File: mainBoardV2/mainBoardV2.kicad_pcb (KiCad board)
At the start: 2 copper layers, 41.1 x 40.7 mm, 30 parts, among them J1 USB4125-GF-A_REVA2, U3 MCP73871-2AAI_ML, U4 MPU6050_Module, U5 TPS61023DRLT

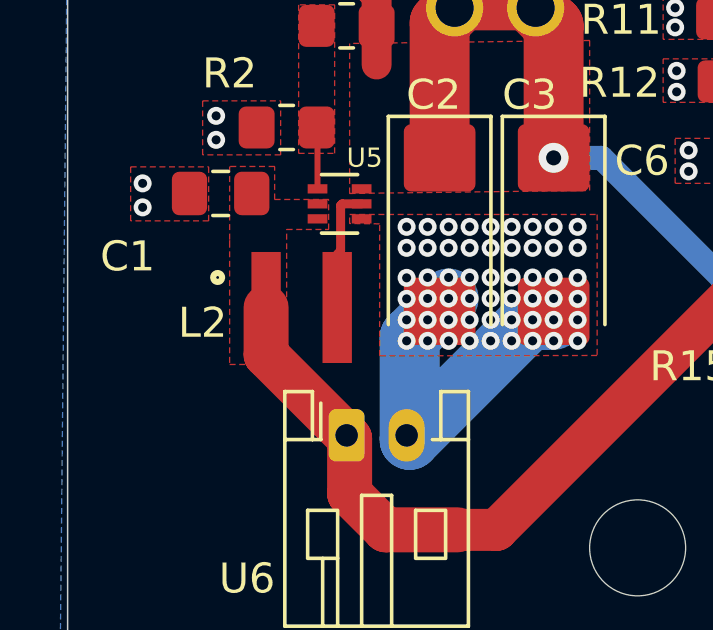
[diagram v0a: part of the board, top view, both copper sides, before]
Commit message: Revert "3.22.26.C1"
This reverts commit 781c2ef683714b83309e94a3ccc7edb13d8085a7.
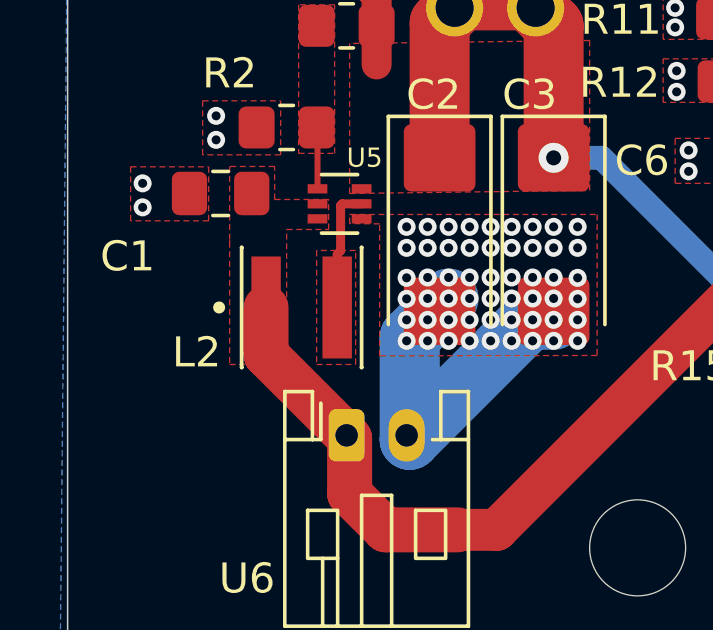
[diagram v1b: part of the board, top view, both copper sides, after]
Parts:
- L2: footprint WE-MAPI_4030:WE-MAPI_4030 -> XEL4030-102MEC:IND_XEL4030-102MEC
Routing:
- net /SW: track 2.40 -> 4.17 mm
- added copper zone on F.Cu, net /SW
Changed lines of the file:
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@@
 		(pcbplotparams
 			(layerselection 0x00000000_00000000_55555555_5755f5ff)
-			(plot_on_all_layers_selection 0x00000000_00000000_00000000_0200000c)
+			(plot_on_all_layers_selection 0x00000000_00000000_00000000_00000000)
 			(disableapertmacros no)
 			(usegerberextensions yes)
@@
 			(drillshape 0)
 			(scaleselection 1)
-			(outputdirectory "C:/Users/edwin/Documents/GitHub/mainBoardProject/mainBoardV2/fabricationFiles2/")
+			(outputdirectory "fabricationFiles/")
 		)
 	)
@@
 		(embedded_fonts no)
 	)
-	(footprint "WE-MAPI_4030:WE-MAPI_4030"
+	(footprint "XEL4030-102MEC:IND_XEL4030-102MEC"
 		(layer "F.Cu")
 		(at 208.4 127.6875)
 		(property "Reference" "L2"
-			(at -3.3 0.5125 0)
+			(at -3.5 1.5 0)
 			(layer "F.SilkS")
 			(effects
@@
 		)
 		(property "Value" "XEL4030-102MEC"
-			(at 0 3.365 0)
+			(at 8.43 3.135 0)
 			(layer "F.Fab")
 			(effects
@@
 		(sheetfile "mainBoardV2.kicad_sch")
 		(attr smd)
+		(fp_line
+			(start -2 -2)
+			(end -1.995 -2)
+			(stroke
+				(width 0.127)
+				(type solid)
+			)
+			(layer "F.SilkS")
+		)
+		(fp_line
+			(start -2 2)
+			(end -2 -2)
+			(stroke
+				(width 0.127)
+				(type solid)
+			)
+			(layer "F.SilkS")
+		)
+		(fp_line
+			(start -1.995 2)
+			(end -2 2)
+			(stroke
+				(width 0.127)
+				(type solid)
+			)
+			(layer "F.SilkS")
+		)
+		(fp_line
+			(start 1.995 -2)
+			(end 2 -2)
+			(stroke
+				(width 0.127)
+				(type solid)
+			)
+			(layer "F.SilkS")
+		)
+		(fp_line
+			(start 2 -2)
+			(end 2 2)
+			(stroke
+				(width 0.127)
+				(type solid)
+			)
+			(layer "F.SilkS")
+		)
+		(fp_line
+			(start 2 2)
+			(end 1.995 2)
+			(stroke
+				(width 0.127)
+				(type solid)
+			)
+			(layer "F.SilkS")
+		)
 		(fp_circle
-			(center -2.8 -1)
-			(end -2.7 -1)
+			(center -2.75 0)
+			(end -2.65 0)
 			(stroke
-				(width 0.3)
+				(width 0.2)
 				(type solid)
 			)
@@
 			(layer "F.SilkS")
 		)
-		(fp_poly
-			(pts
-				(xy -2.35 -2.35) (xy 2.35 -2.35) (xy 2.35 2.35) (xy -2.35 2.35)
-			)
+		(fp_line
+			(start -2.25 -2.25)
+			(end -2.25 2.25)
 			(stroke
-				(width 0.1)
+				(width 0.05)
 				(type solid)
 			)
-			(fill yes)
 			(layer "F.CrtYd")
 		)
 		(fp_line
-			(start -2.15 -2.15)
-			(end 2.15 -2.15)
+			(start -2.25 2.25)
+			(end 2.25 2.25)
 			(stroke
-				(width 0.2)
+				(width 0.05)
 				(type solid)
 			)
-			(layer "F.Fab")
+			(layer "F.CrtYd")
 		)
 		(fp_line
-			(start -2.15 2.15)
-			(end -2.15 -2.15)
+			(start 2.25 -2.25)
+			(end -2.25 -2.25)
 			(stroke
-				(width 0.2)
+				(width 0.05)
 				(type solid)
 			)
-			(layer "F.Fab")
+			(layer "F.CrtYd")
 		)
 		(fp_line
-			(start -2.05 -2.05)
-			(end 2.05 -2.05)
+			(start 2.25 2.25)
+			(end 2.25 -2.25)
 			(stroke
-				(width 0.1)
+				(width 0.05)
 				(type solid)
 			)
-			(layer "F.Fab")
+			(layer "F.CrtYd")
 		)
 		(fp_line
-			(start -2.05 2.05)
-			(end -2.05 -2.05)
+			(start -2 -2)
+			(end 2 -2)
 			(stroke
-				(width 0.1)
+				(width 0.127)
 				(type solid)
 			)
@@
 		)
 		(fp_line
-			(start 2.05 -2.05)
-			(end 2.05 2.05)
+			(start -2 2)
+			(end -2 -2)
 			(stroke
-				(width 0.1)
+				(width 0.127)
 				(type solid)
 			)
@@
 		)
 		(fp_line
-			(start 2.05 2.05)
-			(end -2.05 2.05)
+			(start 2 -2)
+			(end 2 2)
 			(stroke
-				(width 0.1)
+				(width 0.127)
 				(type solid)
 			)
@@
 		)
 		(fp_line
-			(start 2.15 -2.15)
-			(end 2.15 2.15)
+			(start 2 2)
+			(end -2 2)
 			(stroke
-				(width 0.2)
+				(width 0.127)
 				(type solid)
 			)
 			(layer "F.Fab")
 		)
-		(fp_line
-			(start 2.15 2.15)
-			(end -2.15 2.15)
+		(fp_circle
+			(center -2.75 0)
+			(end -2.65 0)
 			(stroke
 				(width 0.2)
 				(type solid)
 			)
+			(fill no)
 			(layer "F.Fab")
 		)
 		(pad "1" smd rect
 			(at -1.185 0)
-			(size 0.98 3.7)
+			(size 0.98 3.4)
 			(layers "F.Cu" "F.Mask" "F.Paste")
 			(net 13 "/VBatt+")
@@
 		(pad "2" smd rect
 			(at 1.185 0)
-			(size 0.98 3.7)
+			(size 0.98 3.4)
 			(layers "F.Cu" "F.Mask" "F.Paste")
 			(net 6 "/SW")
@@
 	)
 	(segment
+		(start 209.585 125.915)
+		(end 209.585 127.6875)
+		(width 0.3)
+		(layer "F.Cu")
+		(net 6)
+	)
+	(segment
 		(start 210.4 124.2335)
 		(end 209.754 124.2335)
@@
 			)
 		)
+	)
+	(zone
+		(net 6)
+		(net_name "/SW")
+		(layer "F.Cu")
+		(hatch edge 0.5)
+		(connect_pads
+			(clearance 0)
+		)
+		(min_thickness 0.25)
+		(filled_areas_thickness no)
+		(fill yes
+			(thermal_gap 0.5)
+			(thermal_bridge_width 0.5)
+		)
+		(polygon
+			(pts
+				(xy 208.9 125.7875) (xy 208.9 129.5875) (xy 210.2 129.5875) (xy 210.2 125.7875)
+			)
+		)
